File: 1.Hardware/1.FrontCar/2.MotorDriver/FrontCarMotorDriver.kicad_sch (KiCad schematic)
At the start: 10 parts

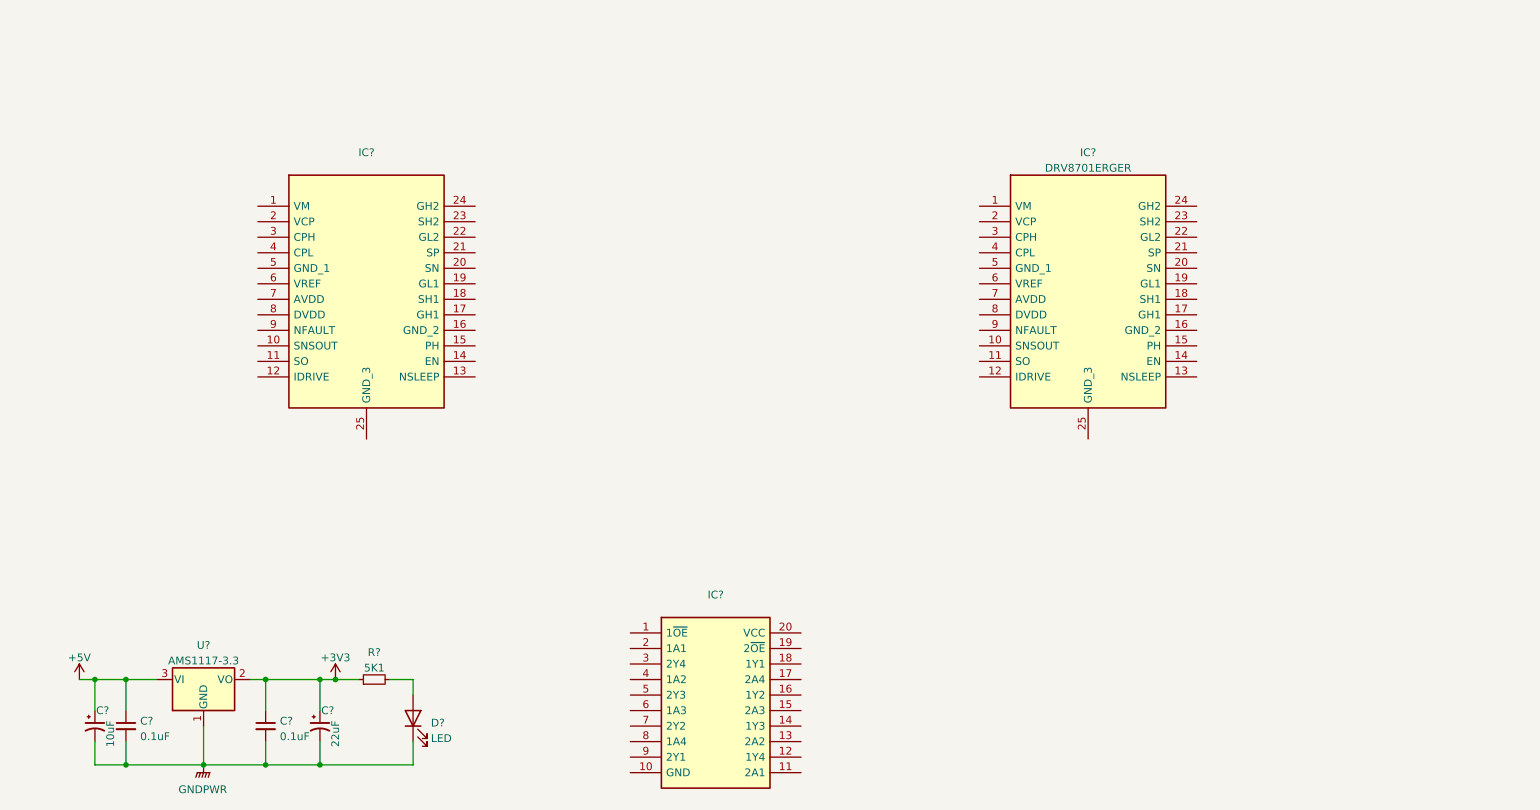
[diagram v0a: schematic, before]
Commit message: drv
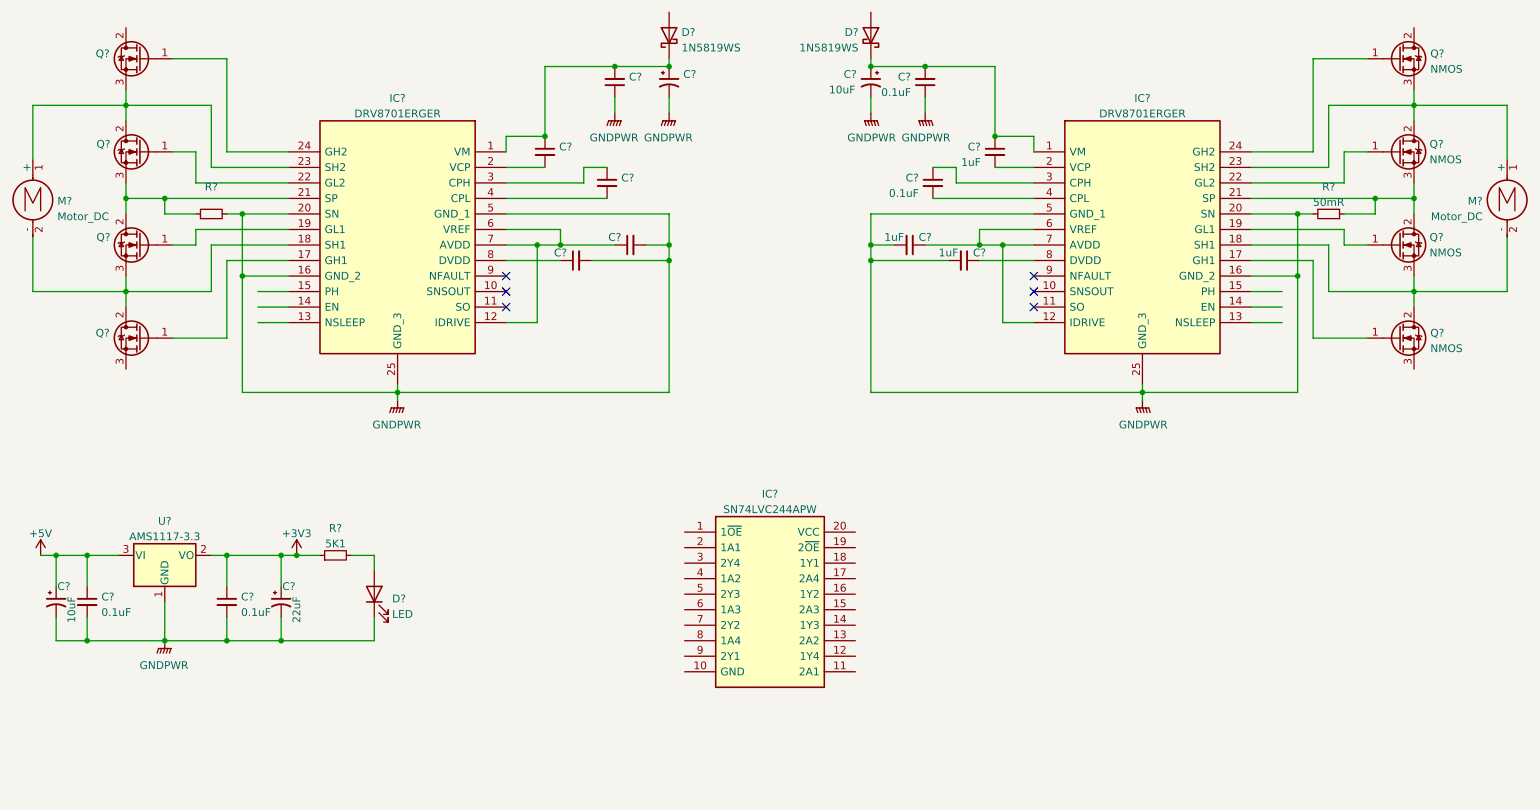
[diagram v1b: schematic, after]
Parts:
- removed IC?: DRV8701ERGER, Package_DFN_QFN:QFN-24-1EP_4x4mm_P0.5mm_EP2.65x2.65mm_ThermalVias, symbol ErBW_s:DRV8701ERGER
- added C? (x3): 1uF, symbol Device:C_Small
- added C?: 10uF, symbol Device:C_Polarized_Small_US
- added C? (x5): (no value), symbol Device:C_Small
- added C? (x2): 0.1uF, symbol Device:C_Small
- added C?: (no value), symbol Device:C_Polarized_Small_US
- added D? (x2): 1N5819WS, Diode_SMD:D_SOD-323, symbol Diode:1N5819WS
- added IC?: DRV8701ERGER, Package_DFN_QFN:QFN-24-1EP_4x4mm_P0.5mm_EP2.65x2.65mm_ThermalVias, symbol ErBW_s:DRV8701ERGER
- added M? (x2): Motor_DC, symbol Motor:Motor_DC
- added Q? (x4): NMOS, ErBW_s:TPH1R403NL, symbol Device:Q_NMOS_GDS
- added Q? (x3): (no value), ErBW_s:TPH1R403NL, symbol Device:Q_NMOS_GDS
- added Q?: (no value), symbol Device:Q_NMOS_GDS
- added R?: (no value), symbol Device:R_Small
- added R?: 50mR, symbol Device:R_Small
- IC?: value (none) -> SN74LVC244APW; footprint (none) -> SOP65P640X120-20N
- IC?: value (none) -> DRV8701ERGER; footprint (none) -> Package_DFN_QFN:QFN-24-1EP_4x4mm_P0.5mm_EP2.65x2.65mm_ThermalVias
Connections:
- net GNDPWR: now also IC?.16 (GND_2), IC?.20 (SN), IC?.25 (GND_3), IC?.5 (GND_1), C?.1, C?.1, C?.2, C?.2, C?.2, C?.2, C?.2, C?.2, IC?.16 (GND_2), IC?.20 (SN), IC?.25 (GND_3), IC?.5 (GND_1), R?.2, R?.2
- net at IC?.1 (VM): now also C?.1, C?.1, C?.2, D?.1 (K)
- net at IC?.12 (IDRIVE): now also IC?.6 (VREF), IC?.7 (AVDD), C?.1
- net at IC?.17 (GH1): now also Q?.1 (G)
- net at IC?.18 (SH1): now also M?.2 (-), Q?.2 (D), Q?.3 (S)
- net at IC?.19 (GL1): now also Q?.1 (G)
- net at IC?.2 (VCP): now also C?.2
- net at IC?.21 (SP): now also Q?.2 (D), Q?.3 (S), R?.1
- net at IC?.22 (GL2): now also Q?.1 (G)
- net at IC?.23 (SH2): now also M?.1 (+), Q?.2 (D), Q?.3 (S)
- net at IC?.24 (GH2): now also Q?.1 (G)
- net at IC?.3 (CPH): now also C?.1
- net at IC?.4 (CPL): now also C?.2
- net at IC?.8 (DVDD): now also C?.1
- new net: C?.1, C?.1, C?.2, D?.1 (K), IC?.1 (VM)
- new net: C?.2, IC?.2 (VCP)
- new net: IC?.23 (SH2), M?.1 (+), Q?.2 (D), Q?.3 (S)
- new net: IC?.18 (SH1), M?.2 (-), Q?.2 (D), Q?.3 (S)
- new net: IC?.19 (GL1), Q?.1 (G)
- new net: IC?.21 (SP), Q?.2 (D), Q?.3 (S), R?.1
- new net: C?.1, IC?.8 (DVDD)
- new net: C?.1, IC?.12 (IDRIVE), IC?.6 (VREF), IC?.7 (AVDD)
- new net: IC?.17 (GH1), Q?.1 (G)
- new net: IC?.22 (GL2), Q?.1 (G)
- new net: IC?.24 (GH2), Q?.1 (G)
- new net: C?.1, IC?.3 (CPH)
- new net: C?.2, IC?.4 (CPL)
- no-connect marks 0 -> 6
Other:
- moved on the sheet: C?, D?, IC?, R?, U?
